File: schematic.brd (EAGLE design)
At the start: 72.4 x 68.2 mm, 7 parts

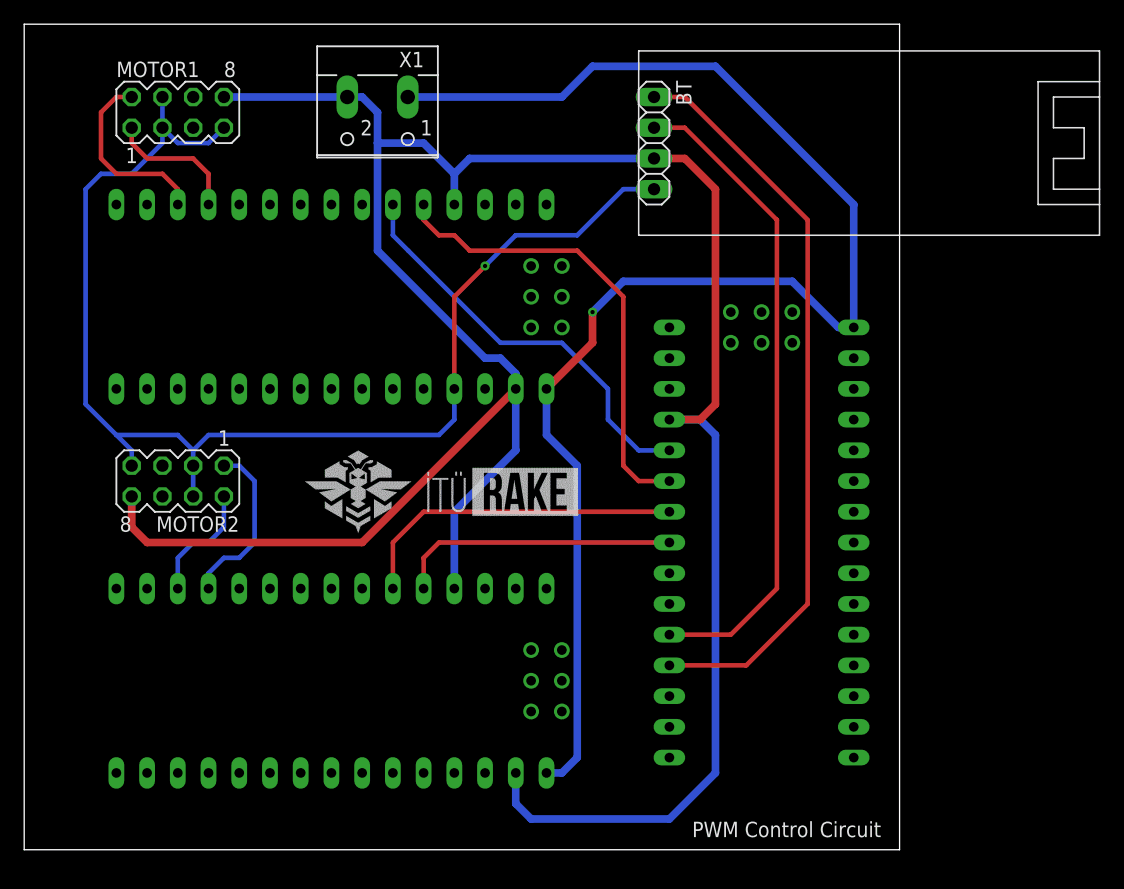
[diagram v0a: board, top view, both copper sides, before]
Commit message: Changes for production
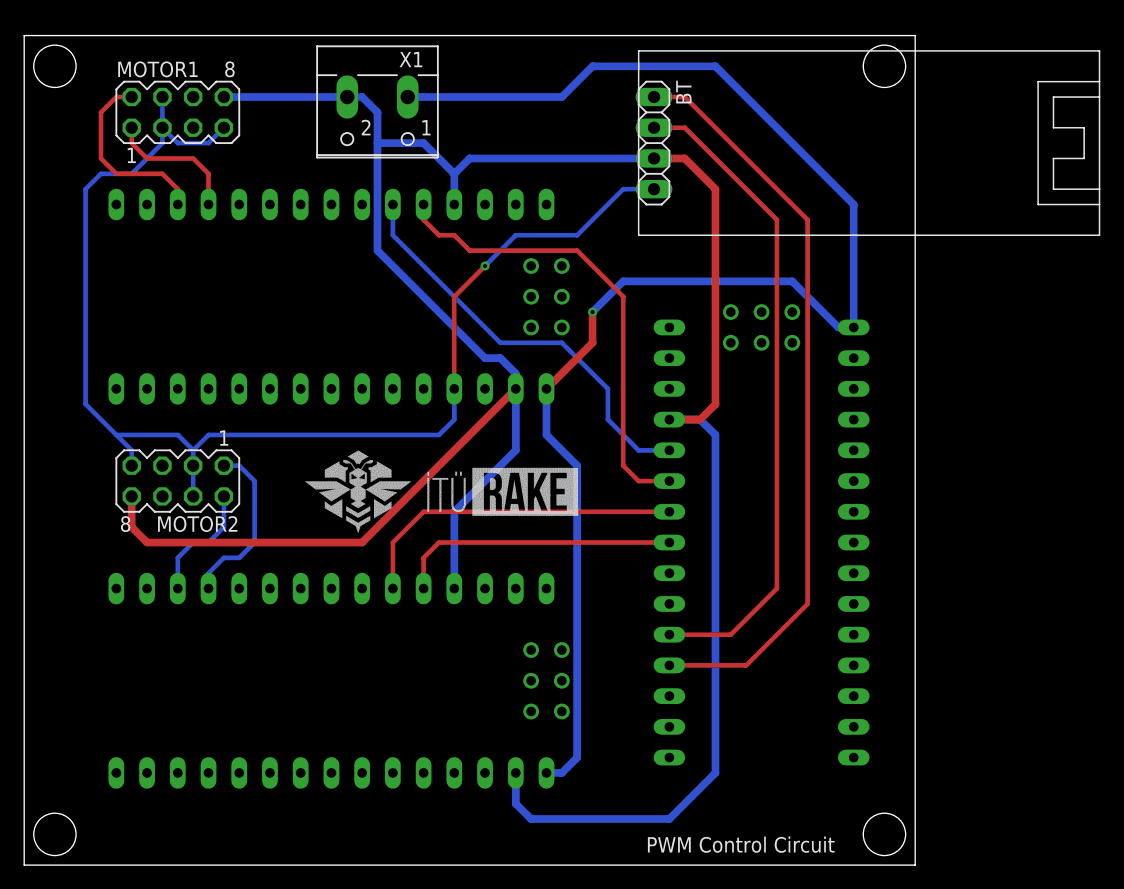
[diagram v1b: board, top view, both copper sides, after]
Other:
- board size 72.4 x 68.2 mm -> 73.7 x 68.6 mm
- board text added: "O.S."
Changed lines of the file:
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@@
 <setting verticaltext="up"/>
 </settings>
-<grid distance="1" unitdist="mil" unit="mil" style="lines" multiple="1" display="yes" altdistance="5" altunitdist="mil" altunit="mil"/>
+<grid distance="1" unitdist="mm" unit="mm" style="lines" multiple="1" display="yes" altdistance="0.05" altunitdist="inch" altunit="inch"/>
 <layers>
 <layer number="1" name="Top" color="4" fill="1" visible="yes" active="yes"/>
@@
 <layer number="43" name="vRestrict" color="2" fill="10" visible="yes" active="yes"/>
 <layer number="44" name="Drills" color="7" fill="1" visible="no" active="yes"/>
-<layer number="45" name="Holes" color="7" fill="1" visible="no" active="yes"/>
+<layer number="45" name="Holes" color="7" fill="1" visible="yes" active="yes"/>
 <layer number="46" name="Milling" color="3" fill="1" visible="no" active="yes"/>
 <layer number="47" name="Measures" color="7" fill="1" visible="no" active="yes"/>
@@
 <board>
 <plain>
-<wire x1="-2.54" y1="8.89" x2="69.83" y2="8.89" width="0" layer="20"/>
-<wire x1="69.83" y1="8.89" x2="69.83" y2="77.14" width="0" layer="20"/>
-<wire x1="69.83" y1="77.14" x2="-2.54" y2="77.14" width="0" layer="20"/>
-<wire x1="-2.54" y1="77.14" x2="-2.54" y2="8.89" width="0" layer="20"/>
+<wire x1="-2.54" y1="7.62" x2="71.12" y2="7.62" width="0" layer="20"/>
+<wire x1="71.12" y1="7.62" x2="71.12" y2="76.2" width="0" layer="20"/>
+<wire x1="71.12" y1="76.2" x2="-2.54" y2="76.2" width="0" layer="20"/>
+<wire x1="-2.54" y1="76.2" x2="-2.54" y2="7.62" width="0" layer="20"/>
 <rectangle x1="25.0571" y1="35.0647" x2="25.0825" y2="35.0901" layer="21"/>
 <rectangle x1="25.0317" y1="35.1155" x2="25.1079" y2="35.1409" layer="21"/>
@@
 <rectangle x1="25.0063" y1="41.8465" x2="25.1333" y2="41.8719" layer="21"/>
 <rectangle x1="25.0571" y1="41.8719" x2="25.0825" y2="41.8973" layer="21"/>
-<text x="52.6796" y="9.9314" size="1.27" layer="21" font="vector">PWM Control Circuit</text>
+<text x="48.8696" y="8.6614" size="1.27" layer="21" font="vector">PWM Control Circuit</text>
+<hole x="0" y="73.66" drill="3.5"/>
+<hole x="68.58" y="73.66" drill="3.5"/>
+<hole x="68.58" y="10.16" drill="3.5"/>
+<hole x="0" y="10.16" drill="3.5"/>
+<text x="8" y="9" size="1.778" layer="22" rot="MR0">O.S.</text>
 </plain>
 <attributes>
